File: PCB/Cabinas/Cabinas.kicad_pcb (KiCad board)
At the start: 2 copper layers, 196.7 x 93.5 mm, 115 parts, among them J1 JACK_ST_3SW, K1 CONN_3, M1 WTV020-SD, P1 CONN_2, P10 CONN_2, P11 CONN_2, P12 CONN_2, P13 DIN_5, P2 CONN_2, P3 CONN_2, P4 CONN_2, P5 CONN_2, P6 CONN_2, P7 CONN_2, P8 CONN_2, P9 CONN_2, Q1 MOSFET_N, Q10 MOSFET_N, Q11 MOSFET_N, Q12 MOSFET_N, Q2 MOSFET_N, Q3 MOSFET_N, Q4 MOSFET_N, Q5 MOSFET_N, Q6 MOSFET_N, Q7 MOSFET_N, Q8 MOSFET_N, Q9 MOSFET_N, SW1 PUSHBUTTON, SW10 PUSHBUTTON, SW11 PUSHBUTTON, SW12 PUSHBUTTON, SW2 PUSHBUTTON, SW3 PUSHBUTTON, SW4 PUSHBUTTON, SW5 PUSHBUTTON, SW6 PUSHBUTTON, SW7 PUSHBUTTON, SW8 PUSHBUTTON, SW9 PUSHBUTTON, U1 BTM, U2 7805, U3 TL072

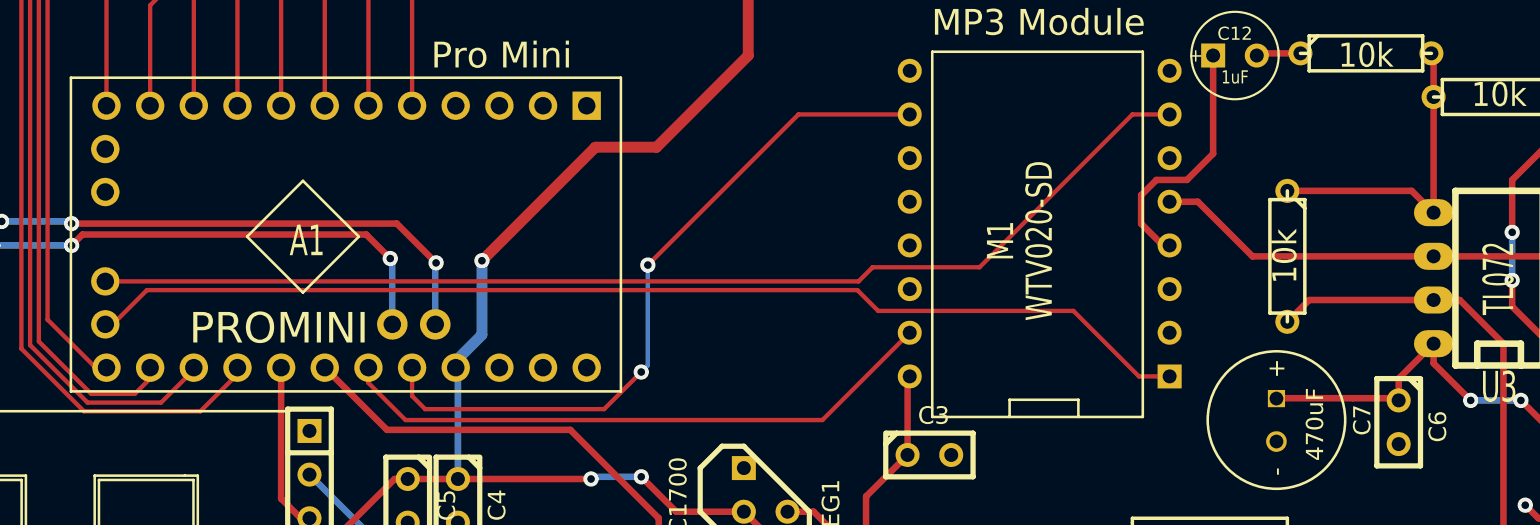
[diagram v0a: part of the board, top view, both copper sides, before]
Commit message: Cambios
Cambio de pines para el módulo MP3
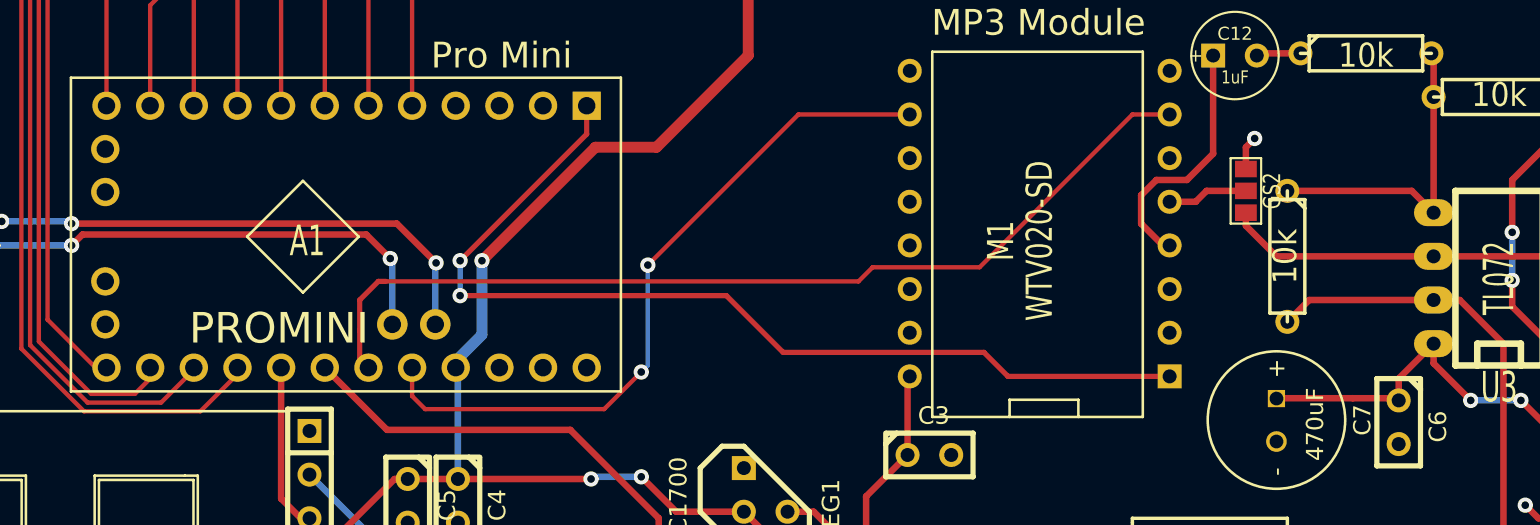
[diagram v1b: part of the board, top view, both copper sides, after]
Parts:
- added GS2: GS3, GS3, F.Cu at (188.5, 121.9)
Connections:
- A1 pad 1: (no net) -> MP3_RESET
- A1 pad 15: MP3_CK -> (no net)
- A1 pad 16: MP3_RESET -> (no net)
- A1 pad 23: MP3_BUSY -> MP3_CK
- ELEC1 pad 4: GND -> (no net)
- ELEC1 pad 6: GND -> (no net)
- M1 pad 15: MP3_BUSY -> (no net)
- M1 pad 5: Vbias -> N-0000055
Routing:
- net MP3_BUSY: track 35.4 -> 0.00 mm
- net MP3_CK: track 65.9 -> 55.7 mm
- net MP3_RESET: track 64.8 -> 57.3 mm, vias 0 -> 2
- net N-0000055: track 0.00 -> 4.70 mm
- net Vbias: track 64.9 -> 60.7 mm
- net GND: track 2.09 -> 4.08 mm, vias 1 -> 2
